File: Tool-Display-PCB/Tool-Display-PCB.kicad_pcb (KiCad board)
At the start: 2 copper layers, 4 parts, among them J1 4" TFT SPI DISPLAY, J2 ESP32 30-Pin

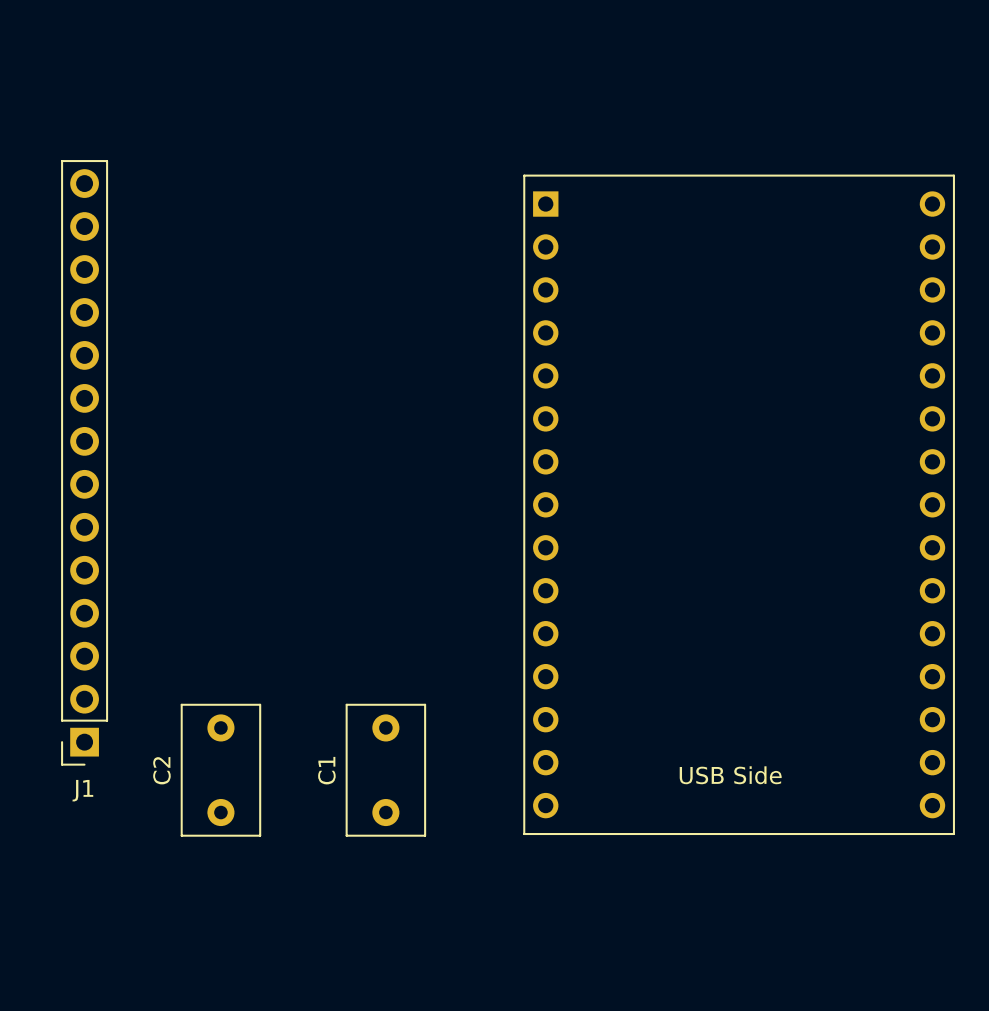
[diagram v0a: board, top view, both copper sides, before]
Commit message: PCB changes
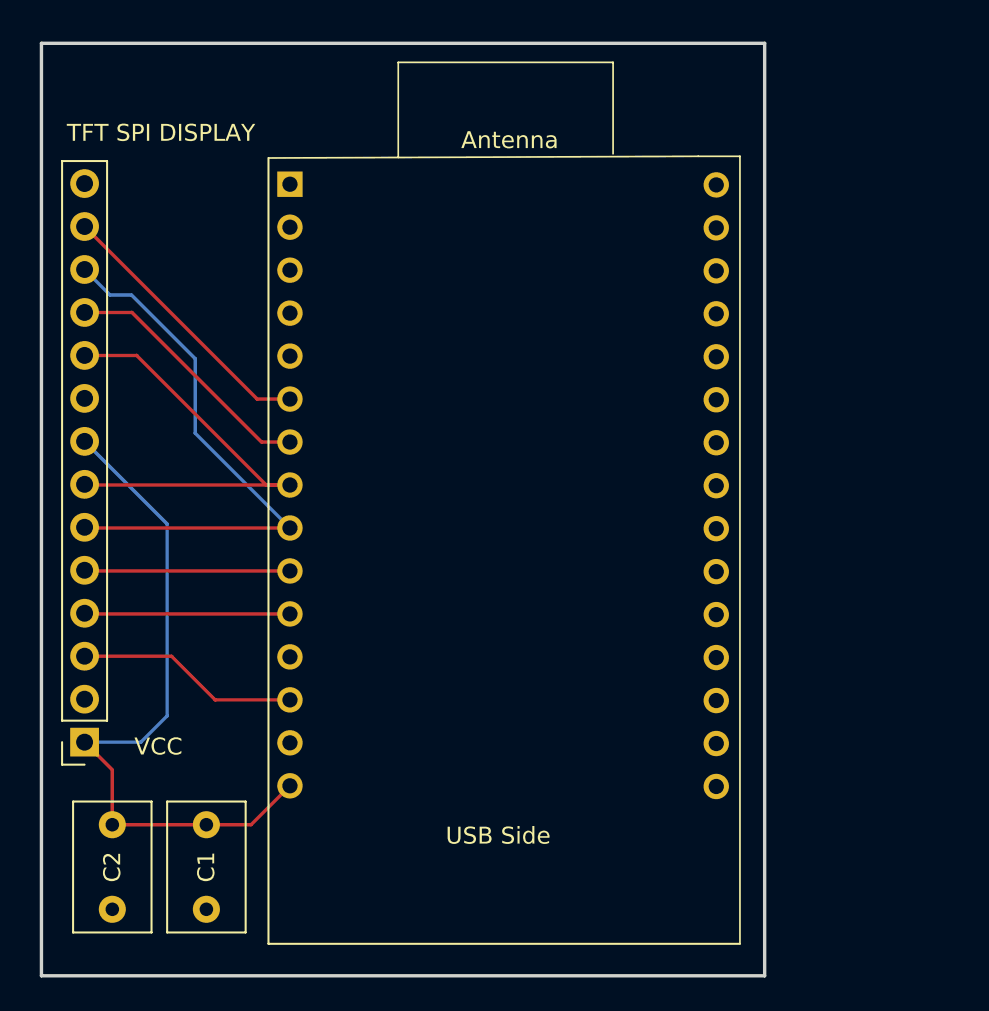
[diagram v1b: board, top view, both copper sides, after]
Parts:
- J1: value 4" TFT SPI DISPLAY -> TFT SPI DISPLAY
- moved J2 15.2 mm to (114.9, 64.7)
- moved C1 12.1 mm to (110.0, 107.5)
- moved C2 8.60 mm to (104.4, 107.5)
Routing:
- net Net-(J1-Pin_1): track 0.00 -> 40.8 mm
- net Net-(J1-Pin_12): track 0.00 -> 33.2 mm
- net Net-(J1-Pin_10): track 0.00 -> 27.5 mm
- net Net-(J2-Pin_10): track 0.00 -> 16.4 mm
- net Net-(J2-Pin_9): track 0.00 -> 15.3 mm
- net Net-(J1-Pin_3): track 0.00 -> 13.2 mm
- net Net-(J1-Pin_5): track 0.00 -> 12.2 mm
- net Net-(J1-Pin_4): track 0.00 -> 12.2 mm
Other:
- board outline added: 42.8 x 55.1 mm
- board text added: "VCC"

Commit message: pcb finished, shipped
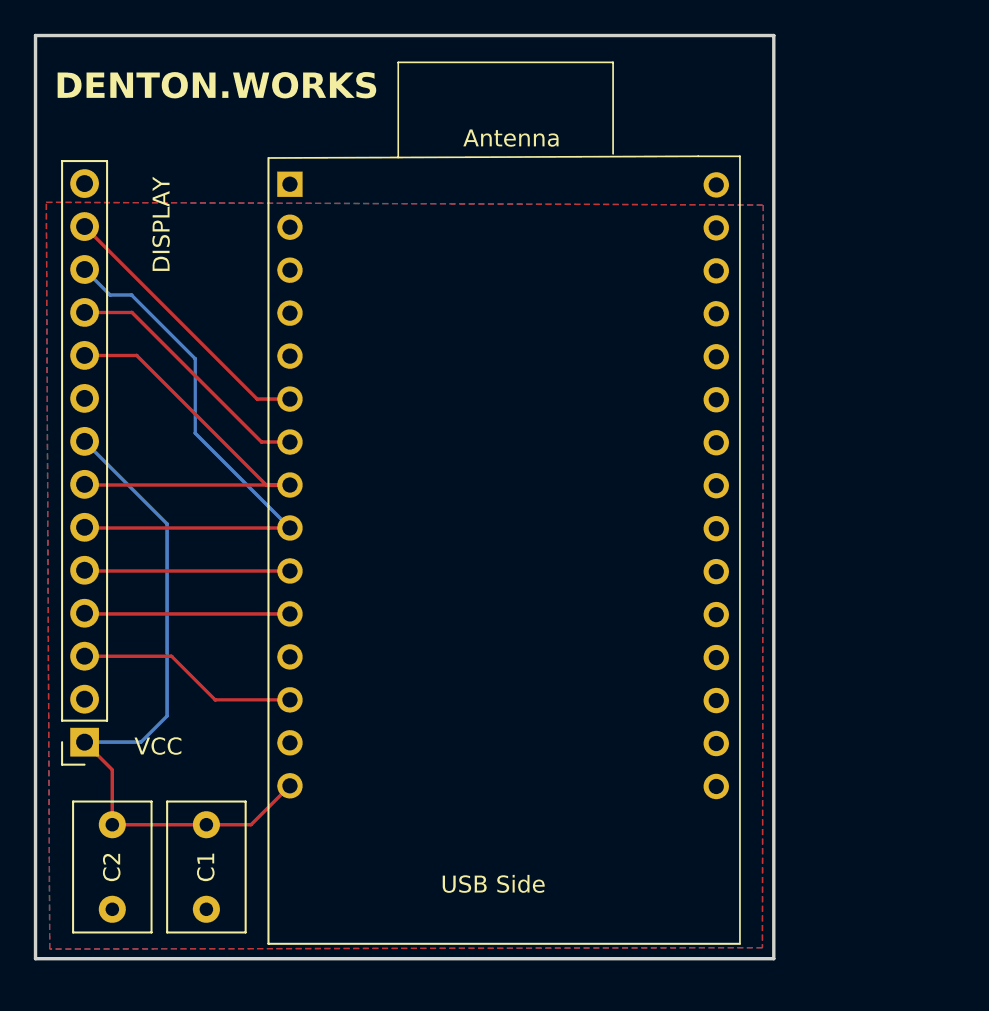
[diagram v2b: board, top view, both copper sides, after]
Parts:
- J1: value TFT SPI DISPLAY -> DISPLAY
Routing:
- added copper zone on B.Cu, net GND
- added copper zone on F.Cu, net GND
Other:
- board size 42.8 x 55.1 mm -> 43.6 x 54.6 mm
- board text added: "DENTON.WORKS"
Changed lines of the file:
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@@
 			(outputformat 1)
 			(mirror no)
-			(drillshape 1)
+			(drillshape 0)
 			(scaleselection 1)
 			(outputdirectory "")
@@
 			)
 		)
-		(property "Value" "TFT SPI DISPLAY"
-			(at -4.52 36.01 0)
+		(property "Value" "DISPLAY"
+			(at -4.56 30.57 90)
 			(layer "F.SilkS")
 			(effects
@@
 		)
 		(fp_text user "USB Side"
-			(at 9.2 39.1 0)
+			(at 8.91 41.99 0)
 			(unlocked yes)
 			(layer "F.SilkS")
@@
 		)
 		(fp_text user "Antenna"
-			(at 13 -2.6 0)
+			(at 13.12 -2.7 0)
 			(unlocked yes)
 			(layer "F.SilkS")
@@
 	)
 	(gr_rect
-		(start 100.24 56.34)
-		(end 142.99 111.46)
+		(start 99.89 55.88)
+		(end 143.53 110.45)
 		(stroke
 			(width 0.2)
@@
 		(fill no)
 		(layer "Edge.Cuts")
+	)
+	(gr_text "DENTON.WORKS"
+		(at 101.01 59.75 0)
+		(layer "F.SilkS")
+		(effects
+			(font
+				(size 1.5 1.5)
+				(thickness 0.3)
+				(bold yes)
+			)
+			(justify left bottom)
+		)
 	)
 	(gr_text "VCC"
@@
 		(net 11)
 	)
+	(zone
+		(net 1)
+		(net_name "GND")
+		(layers "F.Cu" "B.Cu")
+		(hatch edge 0.5)
+		(connect_pads
+			(clearance 0.5)
+		)
+		(min_thickness 0.25)
+		(filled_areas_thickness no)
+		(fill yes
+			(thermal_gap 0.5)
+			(thermal_bridge_width 0.5)
+		)
+		(polygon
+			(pts
+				(xy 100.53 65.74) (xy 142.91 65.9) (xy 142.86 109.8) (xy 100.73 109.88)
+			)
+		)
+	)
 	(embedded_fonts no)
